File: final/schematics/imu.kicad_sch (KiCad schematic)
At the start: 8 parts, among them U1 BMI270, U2 BMI270

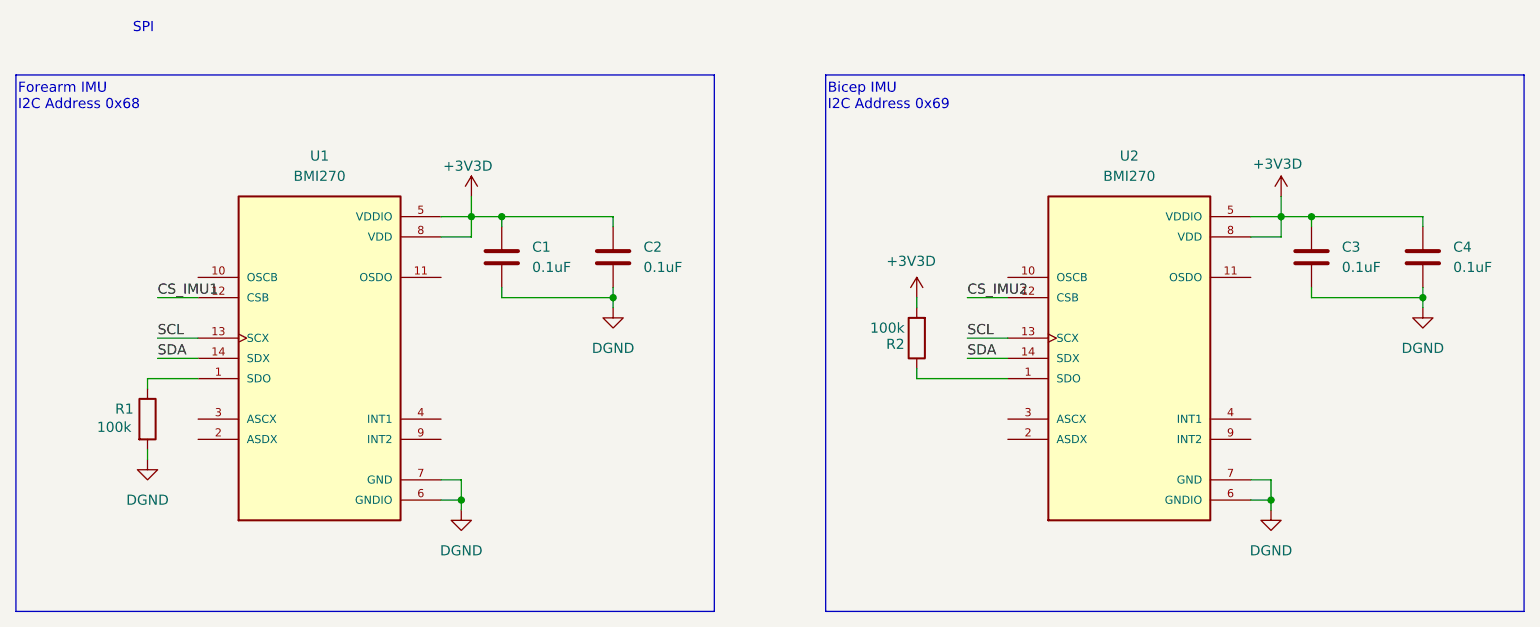
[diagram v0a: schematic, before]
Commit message: finishing
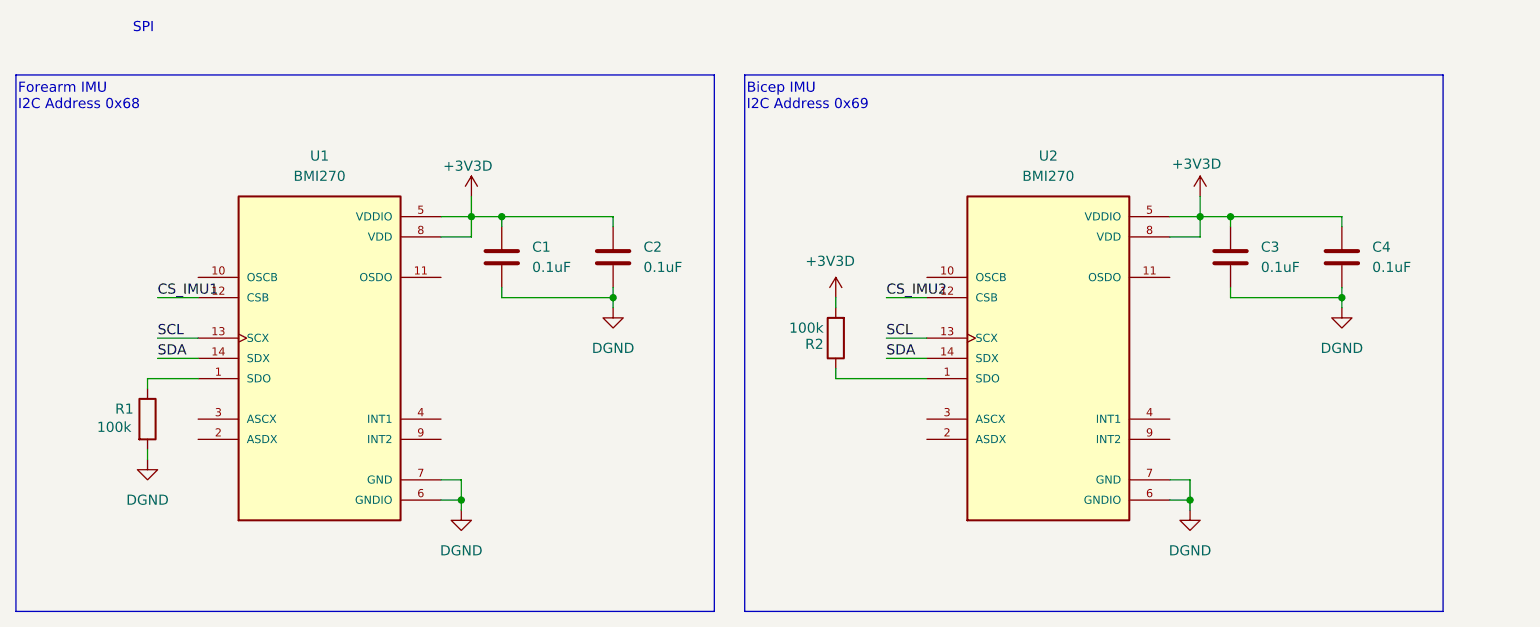
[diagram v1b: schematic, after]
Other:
- moved on the sheet: C3, C4, R2, U2
